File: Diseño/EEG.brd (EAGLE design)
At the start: 49.8 x 80 mm, 42 parts, among them IC1 REF2033AIDDCT, IC2 MCP73831T-2ACI_OT, IC3 LP38692MP-3.3_NOPB, J1 USB3500-30-A-KIT, J2 SJ3-35083A-TR, J3 1769

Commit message: añadido valores cap de carga
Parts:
- C1, C2: value (none) -> 10u
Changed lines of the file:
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@@
 <attribute name="VALUE" x="13.0175" y="34.6075" size="1.27" layer="27" rot="R180" align="center"/>
 </element>
-<element name="C1" library="rcl" library_urn="urn:adsk.eagle:library:334" package="C0805K" package3d_urn="urn:adsk.eagle:package:23681/2" value="" x="22.86" y="22.86" smashed="yes" rot="R180">
+<element name="C1" library="rcl" library_urn="urn:adsk.eagle:library:334" package="C0805K" package3d_urn="urn:adsk.eagle:package:23681/2" value="10u" x="22.86" y="22.86" smashed="yes" rot="R180">
 <attribute name="NAME" x="22.01875" y="20.8775" size="1.016" layer="25"/>
 <attribute name="POPULARITY" value="52" x="-25.4" y="93.98" size="1.778" layer="27" rot="R180" display="off"/>
@@
 <attribute name="VALUE" x="36.195" y="26.67" size="1.27" layer="27" rot="R90"/>
 </element>
-<element name="C2" library="rcl" library_urn="urn:adsk.eagle:library:334" package="C0805K" package3d_urn="urn:adsk.eagle:package:23681/2" value="" x="27.94" y="22.86" smashed="yes">
+<element name="C2" library="rcl" library_urn="urn:adsk.eagle:library:334" package="C0805K" package3d_urn="urn:adsk.eagle:package:23681/2" value="10u" x="27.94" y="22.86" smashed="yes">
 <attribute name="NAME" x="27.09875" y="20.8775" size="1.016" layer="25"/>
 <attribute name="POPULARITY" value="52" x="80.01" y="-48.26" size="1.778" layer="27" display="off"/>

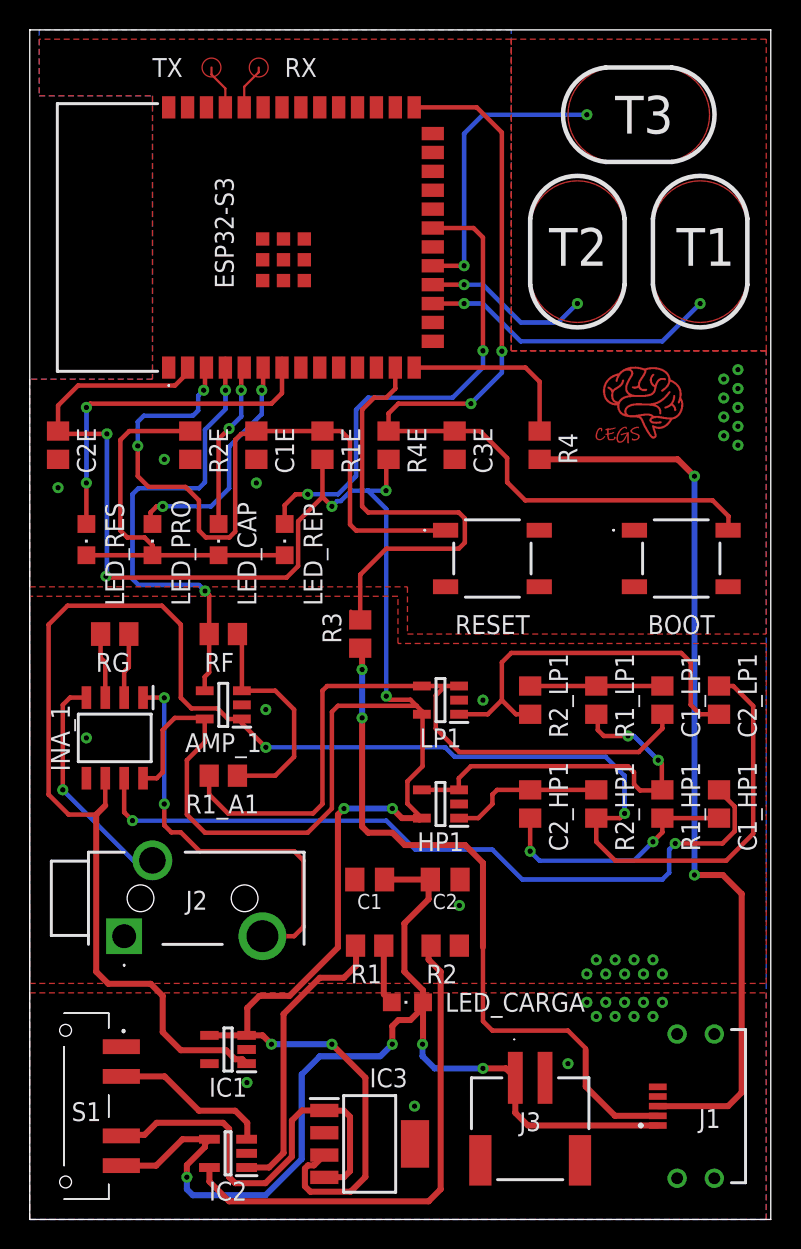
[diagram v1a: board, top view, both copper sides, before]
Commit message: Correcciones del profesor
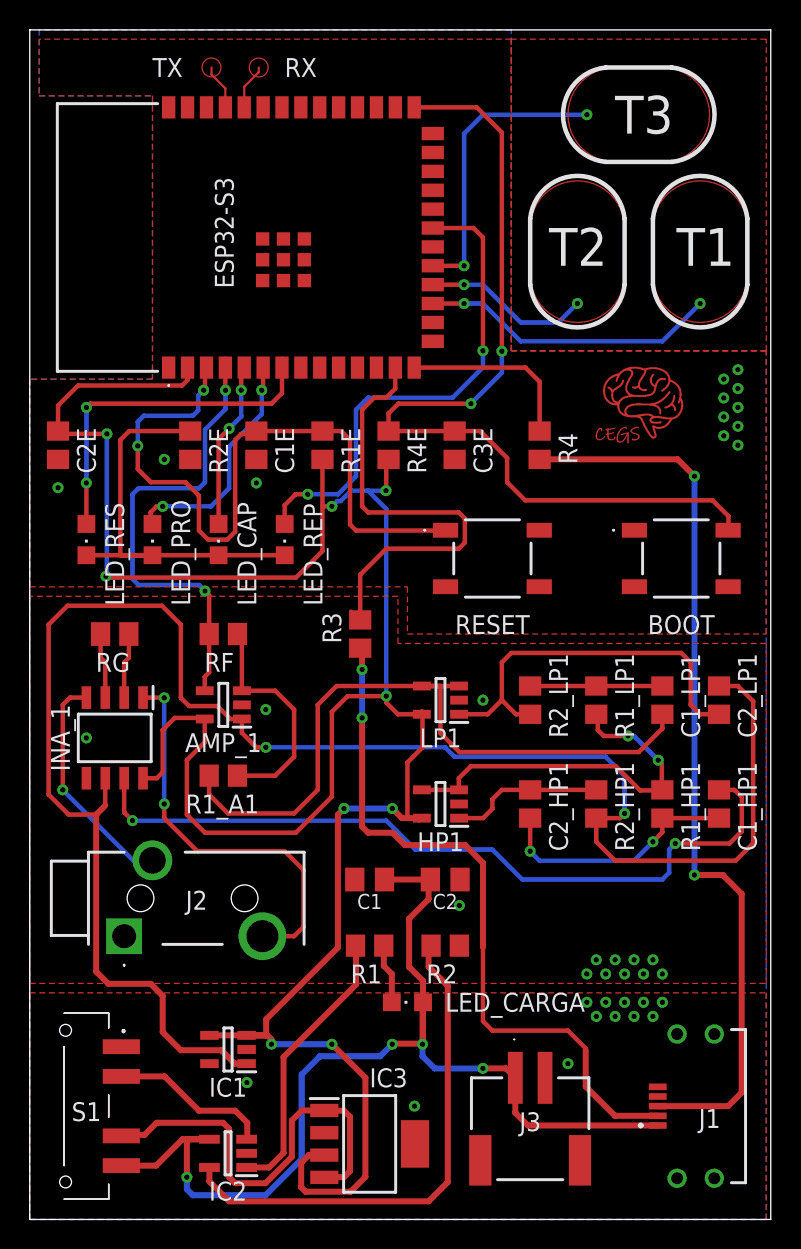
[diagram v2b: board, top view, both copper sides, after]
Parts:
- C1, C2: value 10u -> (none)
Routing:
- net +5V: track 72.0 -> 73.4 mm
- net O1: track 51.2 -> 52.5 mm
- net N$10: track 19.8 -> 18.9 mm
- net VSS: track 119.3 -> 120.3 mm
- net CS1: track 27.8 -> 27.2 mm
- net N$15: track 27.6 -> 28.2 mm
